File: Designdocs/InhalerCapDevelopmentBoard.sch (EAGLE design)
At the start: 23 parts

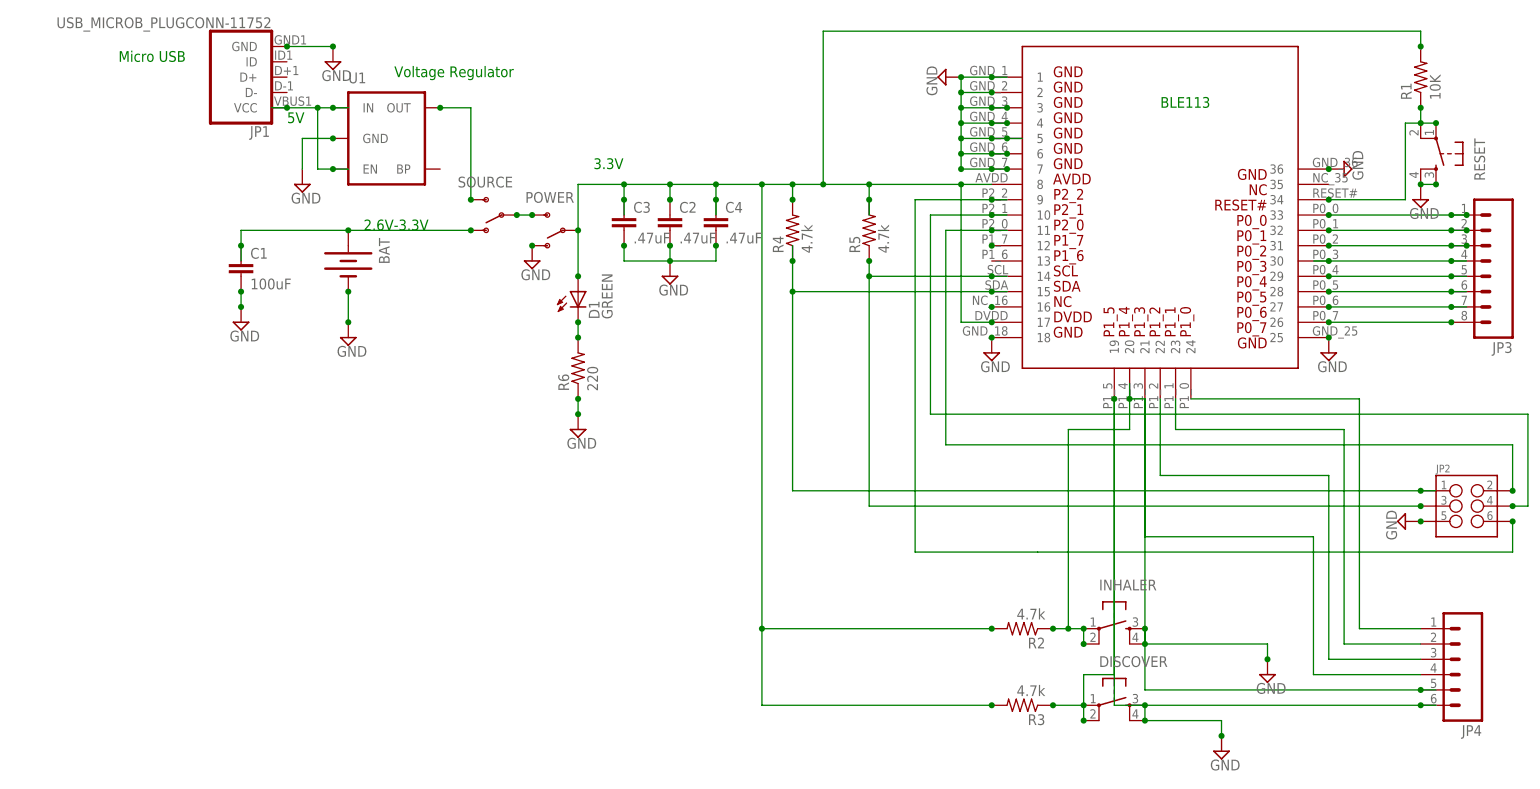
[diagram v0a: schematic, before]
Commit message: Rev. 2 Of Development Board
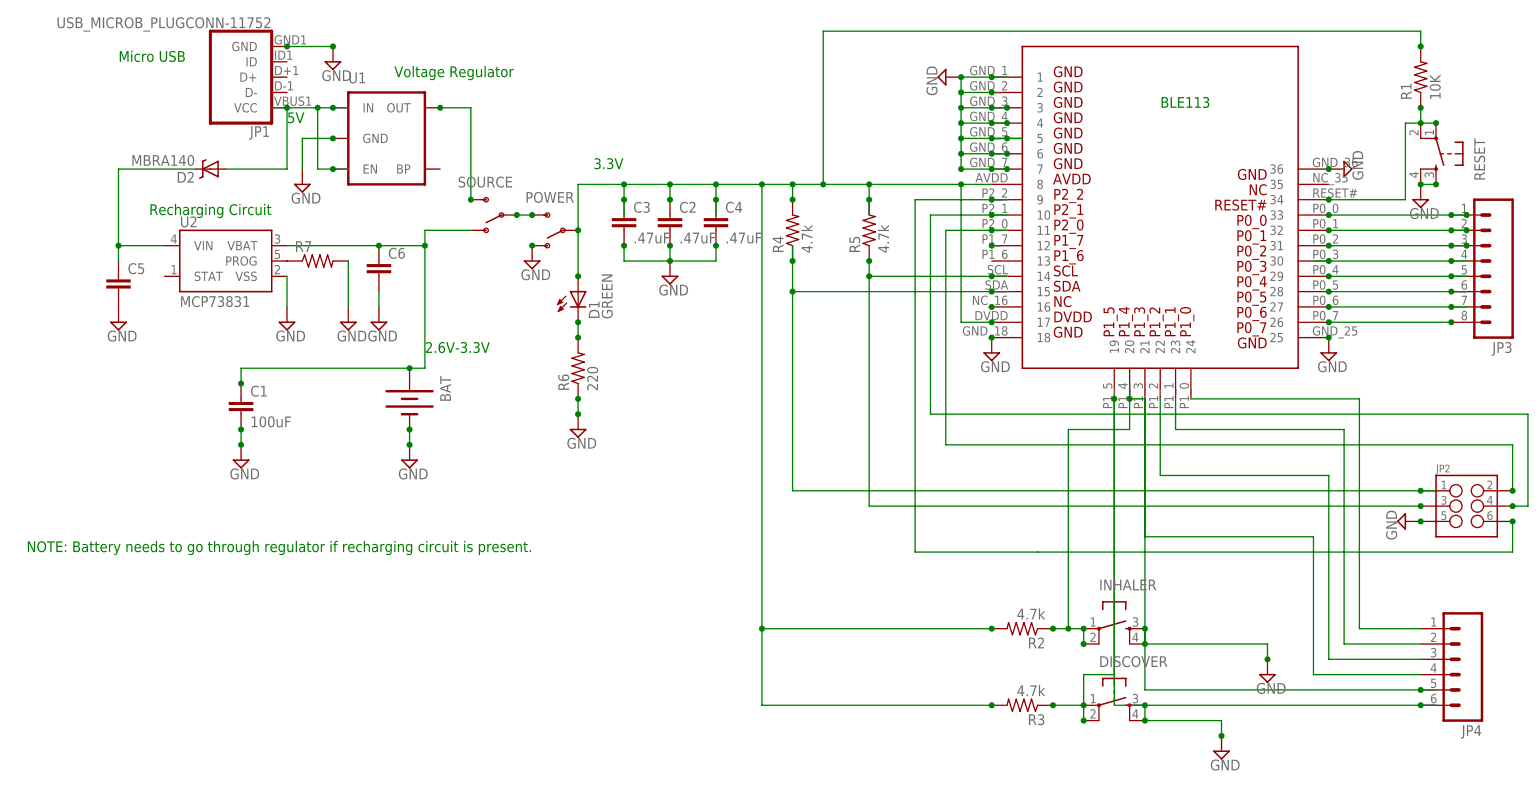
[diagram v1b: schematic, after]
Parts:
- added C5: (no value), SparkFun-Passives:CAP0603-CAP
- added C6: (no value), SparkFun-Capacitors:CAP0603-CAP
- added D2: MBRA140, SparkFun-DiscreteSemi:MBRA140
- added R7: (no value), SparkFun-Passives:RESISTOR0603-RES
- added U2: MCP73831, SparkFun-PowerIC:MCP73831
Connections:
- removed net N$4: BAT.+, C1.1, SOURCE.O
- new net N$29: R7.1, U2.PROG
- new net N$30: C5.1, D2.C, U2.VIN
- new net N$31: BAT.+, C1.1, C6.1, SOURCE.O, U2.VBAT
- net GND: now also C5.2, C6.2, R7.2, U2.VSS
- net N$6: now also D2.A
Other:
- note added: "NOTE: Battery needs to go through regulator if recharging circuit is present."
- note added: "Recharging Circuit"
- moved on the sheet: BAT, C1
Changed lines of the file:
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@@
 <part name="R6" library="SparkFun-Passives" deviceset="RESISTOR" device="0603-RES" value="220"/>
 <part name="JP4" library="SparkFun-Connectors" deviceset="M06" device="NO_SILK"/>
+<part name="D2" library="SparkFun-DiscreteSemi" deviceset="MBRA140" device=""/>
+<part name="C5" library="SparkFun-Passives" deviceset="CAP" device="0603-CAP"/>
+<part name="R7" library="SparkFun-Passives" deviceset="RESISTOR" device="0603-RES"/>
+<part name="U2" library="SparkFun-PowerIC" deviceset="MCP73831" device=""/>
+<part name="C6" library="SparkFun-Capacitors" deviceset="CAP" device="0603-CAP"/>
+<part name="SUPPLY16" library="supply2" deviceset="GND" device=""/>
+<part name="SUPPLY17" library="supply2" deviceset="GND" device=""/>
+<part name="SUPPLY18" library="supply2" deviceset="GND" device=""/>
+<part name="SUPPLY19" library="supply2" deviceset="GND" device=""/>
 </parts>
 <sheets>
@@
 <text x="0" y="106.68" size="1.778" layer="91">5V</text>
 <text x="50.8" y="99.06" size="1.778" layer="91">3.3V</text>
-<text x="12.7" y="88.9" size="1.778" layer="91">2.6V-3.3V</text>
+<text x="22.86" y="68.58" size="1.778" layer="91">2.6V-3.3V</text>
+<text x="-22.86" y="91.44" size="1.778" layer="91">Recharging Circuit</text>
+<text x="-43.18" y="35.56" size="1.778" layer="91">NOTE: Battery needs to go through regulator if recharging circuit is present.</text>
 </plain>
 <instances>
@@
 <instance part="JP1" gate="G$1" x="-7.62" y="114.3" rot="R180"/>
 <instance part="U1" gate="G$1" x="17.78" y="104.14"/>
-<instance part="BAT" gate="G$1" x="10.16" y="83.82" rot="R270"/>
-<instance part="C1" gate="G$1" x="-7.62" y="81.28"/>
+<instance part="BAT" gate="G$1" x="20.32" y="60.96" rot="R270"/>
+<instance part="C1" gate="G$1" x="-7.62" y="58.42"/>
 <instance part="R4" gate="G$1" x="83.82" y="88.9" rot="R90"/>
 <instance part="R5" gate="G$1" x="96.52" y="88.9" rot="R90"/>
@@
 <instance part="SUPPLY1" gate="GND" x="2.54" y="96.52"/>
 <instance part="SUPPLY2" gate="GND" x="7.62" y="116.84"/>
-<instance part="SUPPLY3" gate="GND" x="-7.62" y="73.66"/>
-<instance part="SUPPLY4" gate="GND" x="10.16" y="71.12"/>
+<instance part="SUPPLY3" gate="GND" x="-7.62" y="50.8"/>
+<instance part="SUPPLY4" gate="GND" x="20.32" y="50.8"/>
 <instance part="SUPPLY5" gate="GND" x="63.5" y="81.28"/>
 <instance part="SUPPLY6" gate="GND" x="154.94" y="2.54"/>
@@
 <instance part="R6" gate="G$1" x="48.26" y="66.04" rot="R90"/>
 <instance part="JP4" gate="G$1" x="193.04" y="17.78" rot="R180"/>
+<instance part="D2" gate="G$1" x="-12.7" y="99.06" rot="R180"/>
+<instance part="C5" gate="G$1" x="-27.94" y="78.74"/>
+<instance part="R7" gate="G$1" x="5.08" y="83.82"/>
+<instance part="U2" gate="G$1" x="-10.16" y="83.82"/>
+<instance part="C6" gate="G$1" x="15.24" y="81.28"/>
+<instance part="SUPPLY16" gate="GND" x="-27.94" y="73.66"/>
+<instance part="SUPPLY17" gate="GND" x="0" y="73.66"/>
+<instance part="SUPPLY18" gate="GND" x="10.16" y="73.66"/>
+<instance part="SUPPLY19" gate="GND" x="15.24" y="73.66"/>
 </instances>
 <busses>
@@
 </segment>
 </net>
-<net name="N$4" class="0">
-<segment>
-<wire x1="-7.62" y1="83.82" x2="-7.62" y2="86.36" width="0.1524" layer="91"/>
-<pinref part="SOURCE" gate="1" pin="O"/>
-<wire x1="-7.62" y1="86.36" x2="-7.62" y2="88.9" width="0.1524" layer="91"/>
-<wire x1="-7.62" y1="88.9" x2="10.16" y2="88.9" width="0.1524" layer="91"/>
-<pinref part="BAT" gate="G$1" pin="+"/>
-<junction x="10.16" y="88.9"/>
-<wire x1="10.16" y1="88.9" x2="30.48" y2="88.9" width="0.1524" layer="91"/>
-<junction x="30.48" y="88.9"/>
-<pinref part="C1" gate="G$1" pin="1"/>
-<junction x="-7.62" y="86.36"/>
-</segment>
-</net>
 <net name="N$5" class="0">
 <segment>
@@
 <junction x="7.62" y="99.06"/>
 <junction x="5.08" y="109.22"/>
+<wire x1="0" y1="109.22" x2="0" y2="99.06" width="0.1524" layer="91"/>
+<pinref part="D2" gate="G$1" pin="A"/>
+<wire x1="0" y1="99.06" x2="-10.16" y2="99.06" width="0.1524" layer="91"/>
 </segment>
 </net>
@@
 <segment>
 <pinref part="C1" gate="G$1" pin="2"/>
-<wire x1="-7.62" y1="76.2" x2="-7.62" y2="78.74" width="0.1524" layer="91"/>
+<wire x1="-7.62" y1="53.34" x2="-7.62" y2="55.88" width="0.1524" layer="91"/>
 <pinref part="SUPPLY3" gate="GND" pin="GND"/>
-<junction x="-7.62" y="78.74"/>
-<junction x="-7.62" y="76.2"/>
+<junction x="-7.62" y="55.88"/>
+<junction x="-7.62" y="53.34"/>
 </segment>
 <segment>
 <pinref part="BAT" gate="G$1" pin="-"/>
-<wire x1="10.16" y1="73.66" x2="10.16" y2="78.74" width="0.1524" layer="91"/>
+<wire x1="20.32" y1="53.34" x2="20.32" y2="55.88" width="0.1524" layer="91"/>
 <pinref part="SUPPLY4" gate="GND" pin="GND"/>
-<junction x="10.16" y="78.74"/>
-<junction x="10.16" y="73.66"/>
+<junction x="20.32" y="55.88"/>
+<junction x="20.32" y="53.34"/>
 </segment>
 <segment>
@@
 <junction x="48.26" y="60.96"/>
 </segment>
+<segment>
+<pinref part="C5" gate="G$1" pin="2"/>
+<pinref part="SUPPLY16" gate="GND" pin="GND"/>
+</segment>
+<segment>
+<pinref part="U2" gate="G$1" pin="VSS"/>
+<wire x1="0" y1="81.28" x2="0" y2="76.2" width="0.1524" layer="91"/>
+<pinref part="SUPPLY17" gate="GND" pin="GND"/>
+</segment>
+<segment>
+<pinref part="R7" gate="G$1" pin="2"/>
+<wire x1="10.16" y1="83.82" x2="10.16" y2="76.2" width="0.1524" layer="91"/>
+<pinref part="SUPPLY18" gate="GND" pin="GND"/>
+</segment>
+<segment>
+<pinref part="C6" gate="G$1" pin="2"/>
+<wire x1="15.24" y1="78.74" x2="15.24" y2="76.2" width="0.1524" layer="91"/>
+<pinref part="SUPPLY19" gate="GND" pin="GND"/>
+</segment>
 </net>
 <net name="N$8" class="0">
@@
 </segment>
 </net>
+<net name="N$29" class="0">
+<segment>
+<pinref part="U2" gate="G$1" pin="PROG"/>
+<pinref part="R7" gate="G$1" pin="1"/>
+</segment>
+</net>
+<net name="N$31" class="0">
+<segment>
+<pinref part="BAT" gate="G$1" pin="+"/>
+<wire x1="-7.62" y1="66.04" x2="20.32" y2="66.04" width="0.1524" layer="91"/>
+<wire x1="-7.62" y1="63.5" x2="-7.62" y2="66.04" width="0.1524" layer="91"/>
+<pinref part="C1" gate="G$1" pin="1"/>
+<junction x="-7.62" y="63.5"/>
+<pinref part="U2" gate="G$1" pin="VBAT"/>
+<pinref part="C6" gate="G$1" pin="1"/>
+<wire x1="0" y1="86.36" x2="15.24" y2="86.36" width="0.1524" layer="91"/>
+<wire x1="15.24" y1="86.36" x2="22.86" y2="86.36" width="0.1524" layer="91"/>
+<wire x1="22.86" y1="86.36" x2="22.86" y2="88.9" width="0.1524" layer="91"/>
+<junction x="15.24" y="86.36"/>
+<pinref part="SOURCE" gate="1" pin="O"/>
+<wire x1="22.86" y1="88.9" x2="30.48" y2="88.9" width="0.1524" layer="91"/>
+<wire x1="20.32" y1="66.04" x2="22.86" y2="66.04" width="0.1524" layer="91"/>
+<wire x1="22.86" y1="66.04" x2="22.86" y2="86.36" width="0.1524" layer="91"/>
+<junction x="20.32" y="66.04"/>
+<junction x="22.86" y="86.36"/>
+</segment>
+</net>
+<net name="N$30" class="0">
+<segment>
+<pinref part="C5" gate="G$1" pin="1"/>
+<wire x1="-27.94" y1="83.82" x2="-27.94" y2="86.36" width="0.1524" layer="91"/>
+<pinref part="U2" gate="G$1" pin="VIN"/>
+<wire x1="-27.94" y1="86.36" x2="-20.32" y2="86.36" width="0.1524" layer="91"/>
+<wire x1="-27.94" y1="86.36" x2="-27.94" y2="99.06" width="0.1524" layer="91"/>
+<junction x="-27.94" y="86.36"/>
+<pinref part="D2" gate="G$1" pin="C"/>
+<wire x1="-27.94" y1="99.06" x2="-15.24" y2="99.06" width="0.1524" layer="91"/>
+</segment>
+</net>
